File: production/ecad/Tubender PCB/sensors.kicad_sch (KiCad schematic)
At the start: 6 parts, among them J10 1729157, J11 1729157, J12 1729160, J13 1729131, J8 1729160, J9 1729160

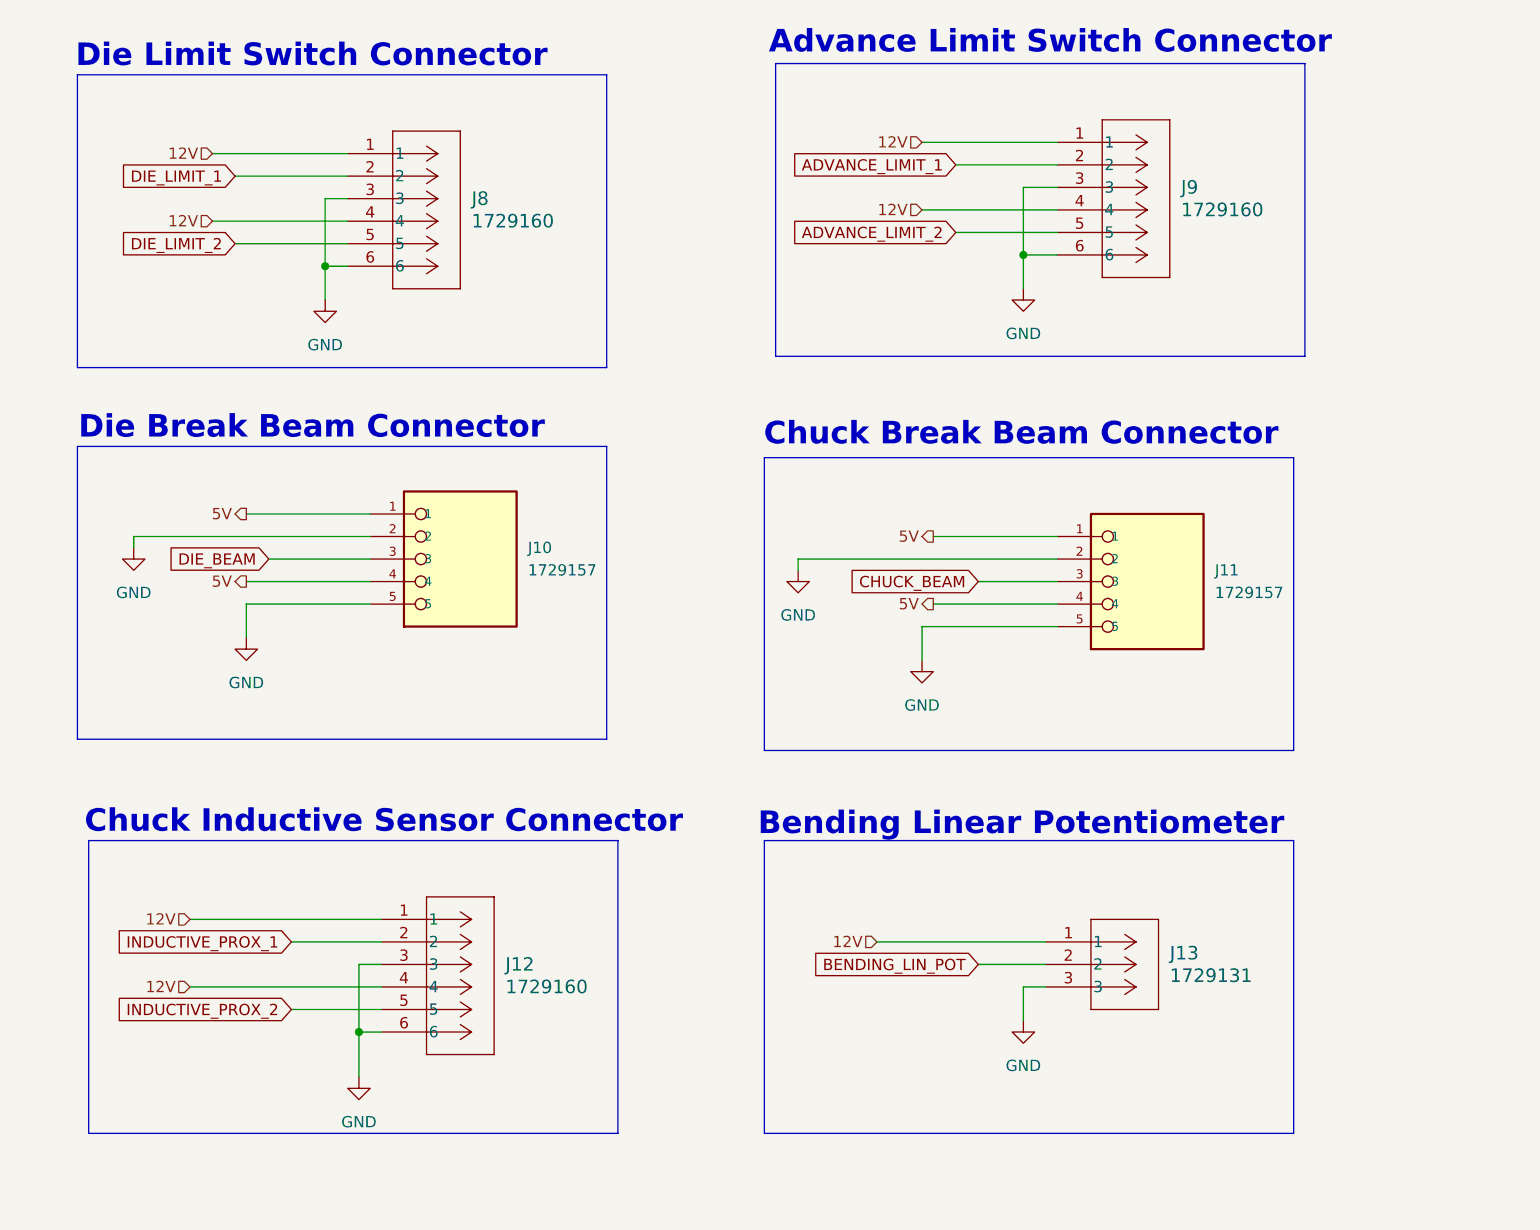
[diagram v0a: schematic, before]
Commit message: Formatting
Boom
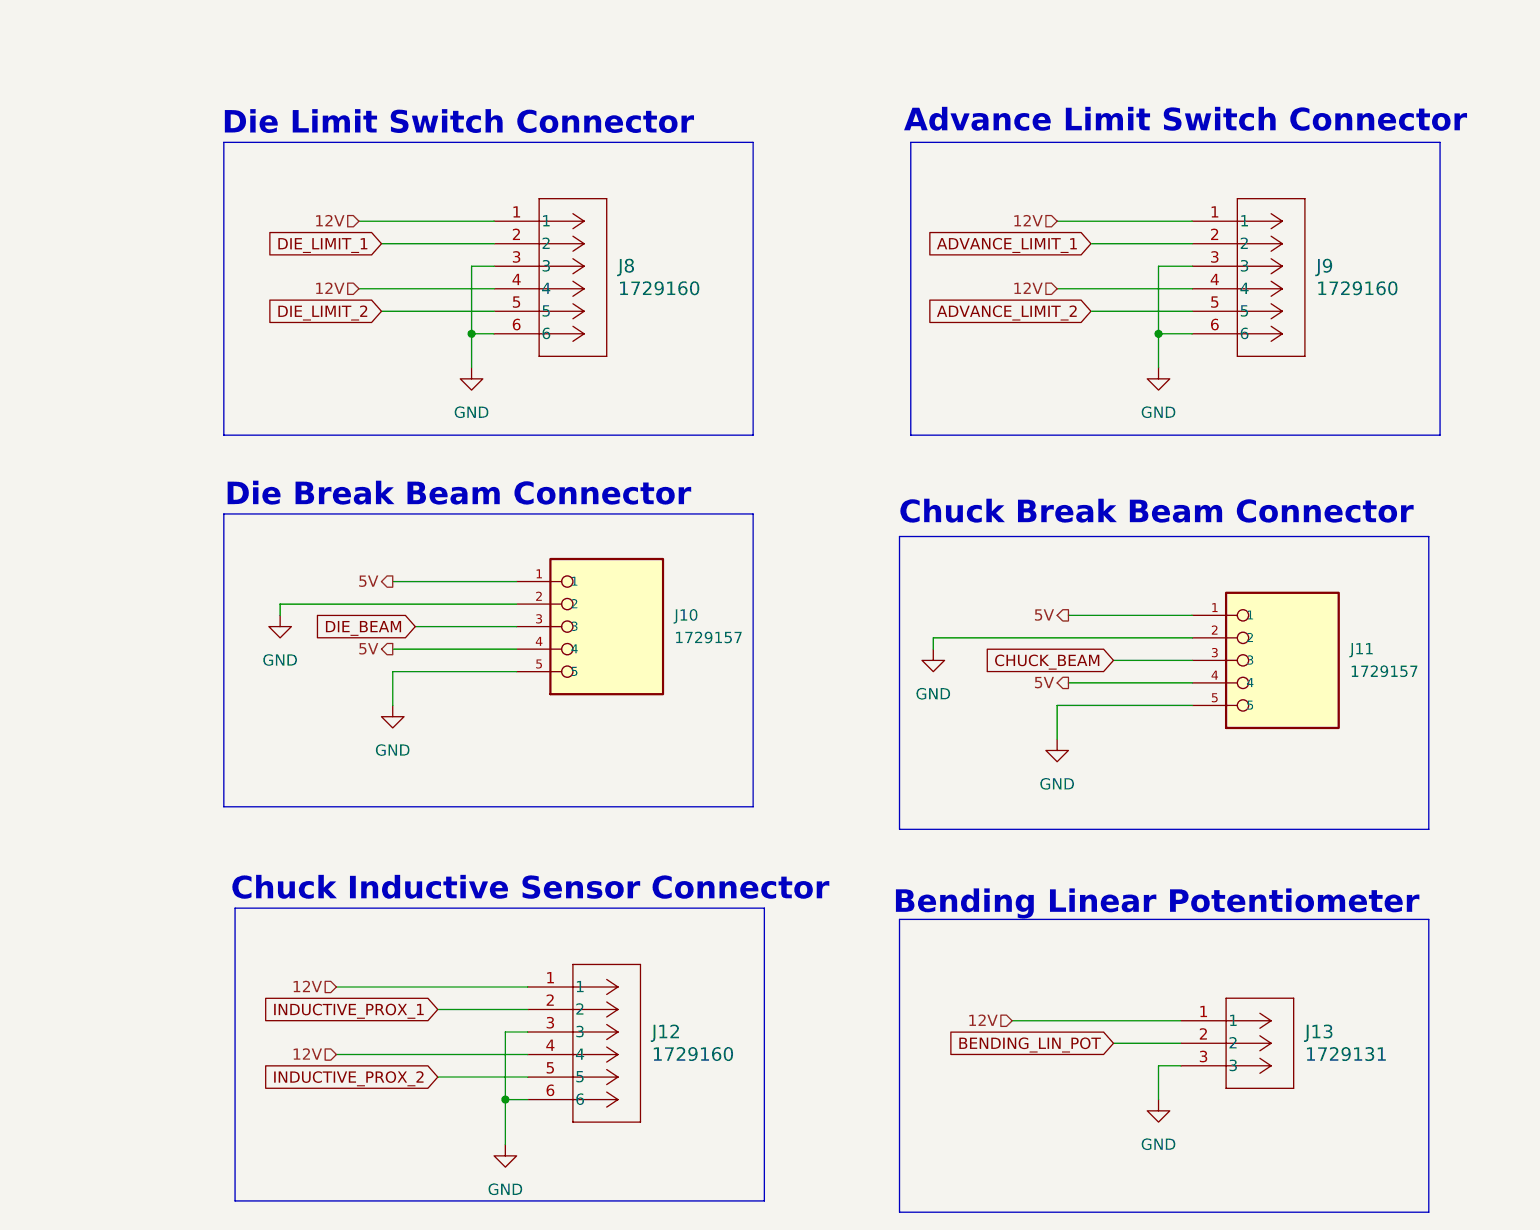
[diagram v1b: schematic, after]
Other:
- moved on the sheet: J10, J11, J12, J13, J8, J9

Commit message: final for rev 1
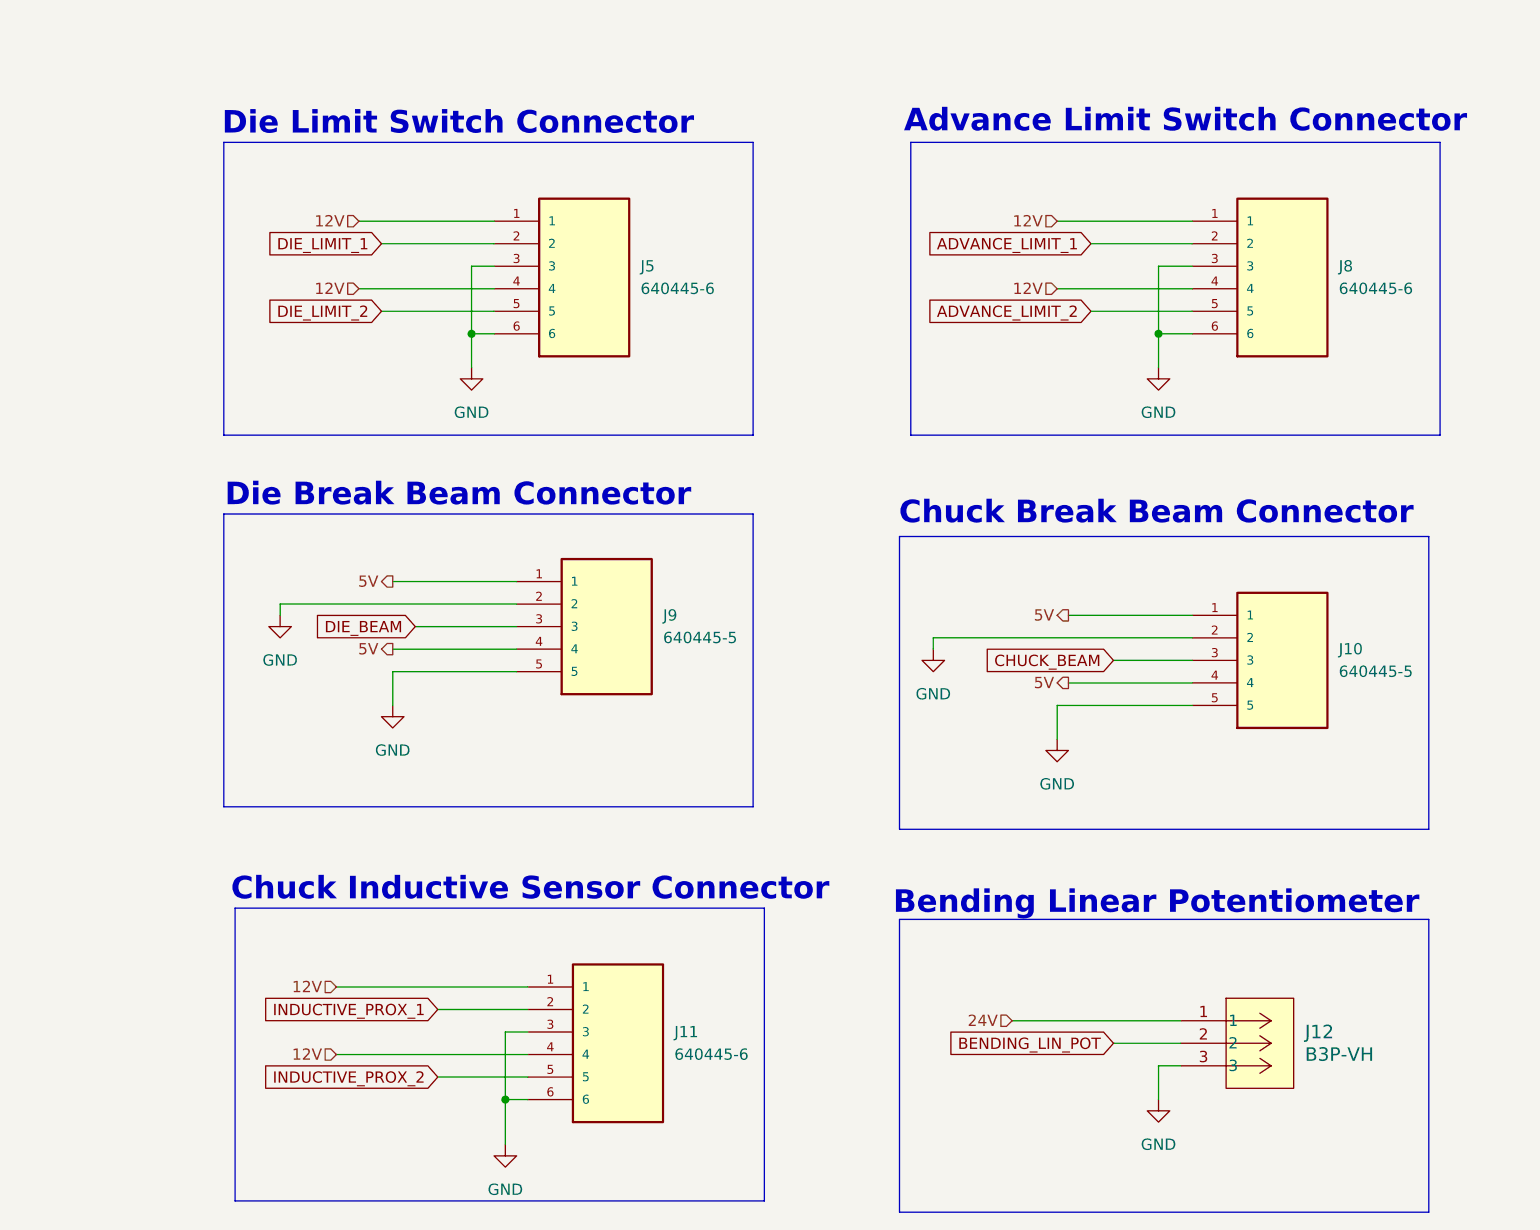
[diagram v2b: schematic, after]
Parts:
- removed J10, J11: 1729157, 1729157:PHOENIX_1729157, symbol 1729157:1729157
- removed J12, J8, J9: 1729160, CONN_1729160_PXC, symbol 1729160:1729160
- removed J13: 1729131, CONN_1729131_PXC, symbol 1729131:1729131
- added J10, J9: 640445-5, 640445-5:TE_640445-5, symbol 640445-5:640445-5
- added J11, J5, J8: 640445-6, 640445-6:TE_640445-6, symbol 640445-6:640445-6
- added J12: B3P-VH, CONN3X1_B3P-VH_JST, symbol 2024-10-11_08-07-43:B3P-VH
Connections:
- net 12V: now also J11.1, J11.4, J5.1, J5.4, J8.1, J8.4
- net 5V: now also J10.1, J10.4, J9.1, J9.4
- net ADVANCE_LIMIT_1: now also J8.2
- net ADVANCE_LIMIT_2: now also J8.5
- net BENDING_LIN_POT: now also J12.2
- net CHUCK_BEAM: now also J10.3
- net DIE_BEAM: now also J9.3
- net DIE_LIMIT_1: now also J5.2
- net DIE_LIMIT_2: now also J5.5
- net GND: now also J10.2, J10.5, J11.3, J11.6, J12.3, J5.3, J5.6, J8.3, J8.6, J9.2, J9.5
- net INDUCTIVE_PROX_1: now also J11.2
- net INDUCTIVE_PROX_2: now also J11.5
- new net 24V: J12.1
